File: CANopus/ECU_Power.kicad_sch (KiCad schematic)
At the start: 1 part

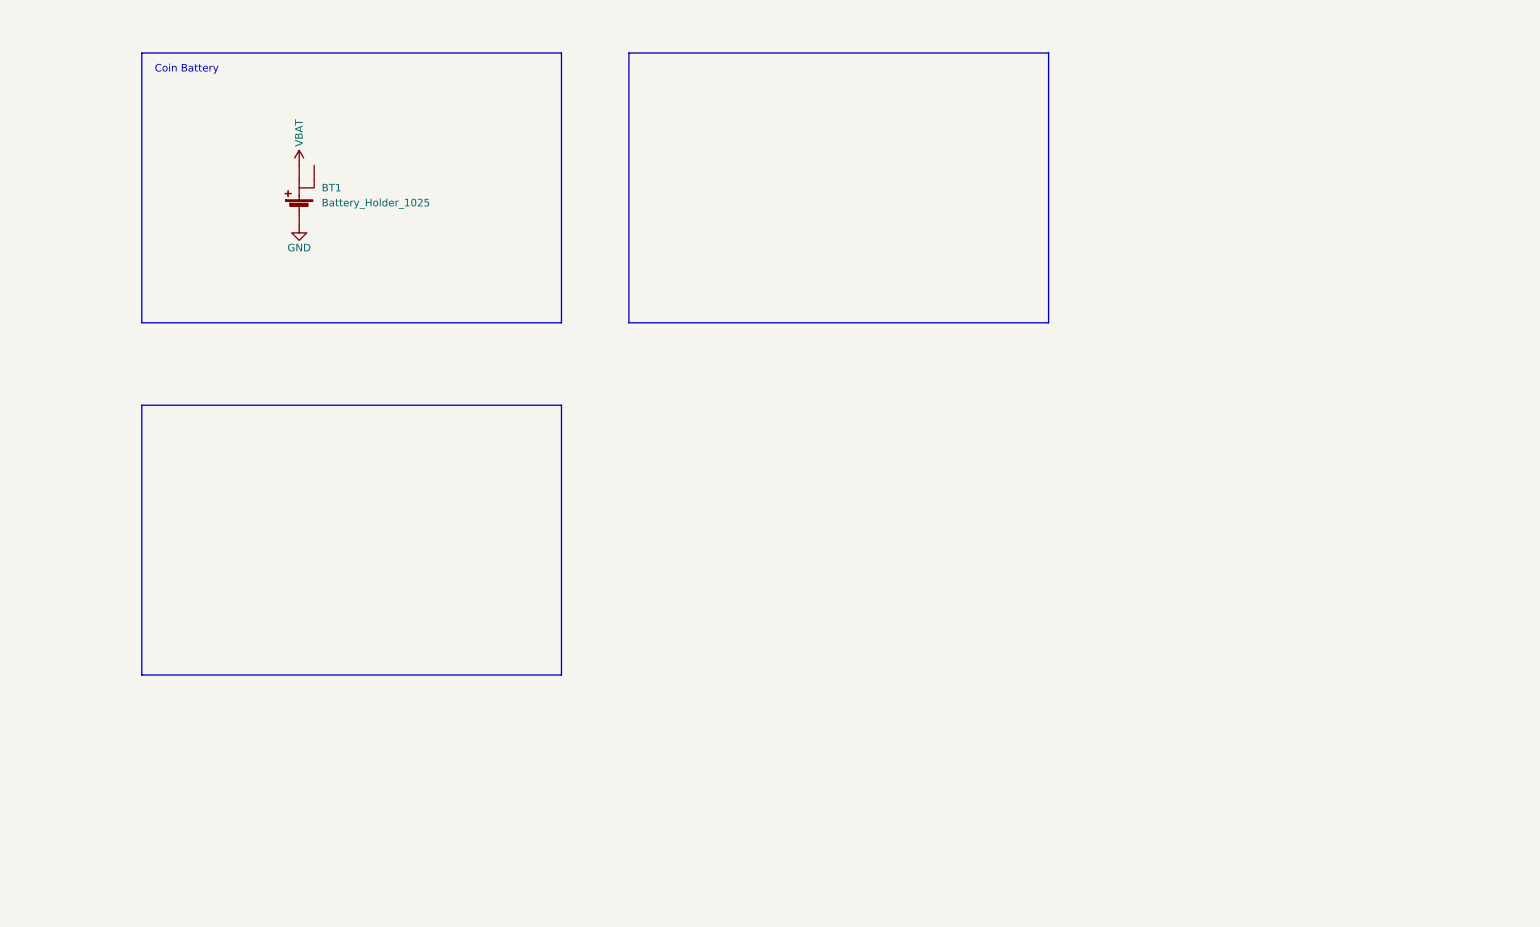
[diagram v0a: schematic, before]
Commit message: Alim
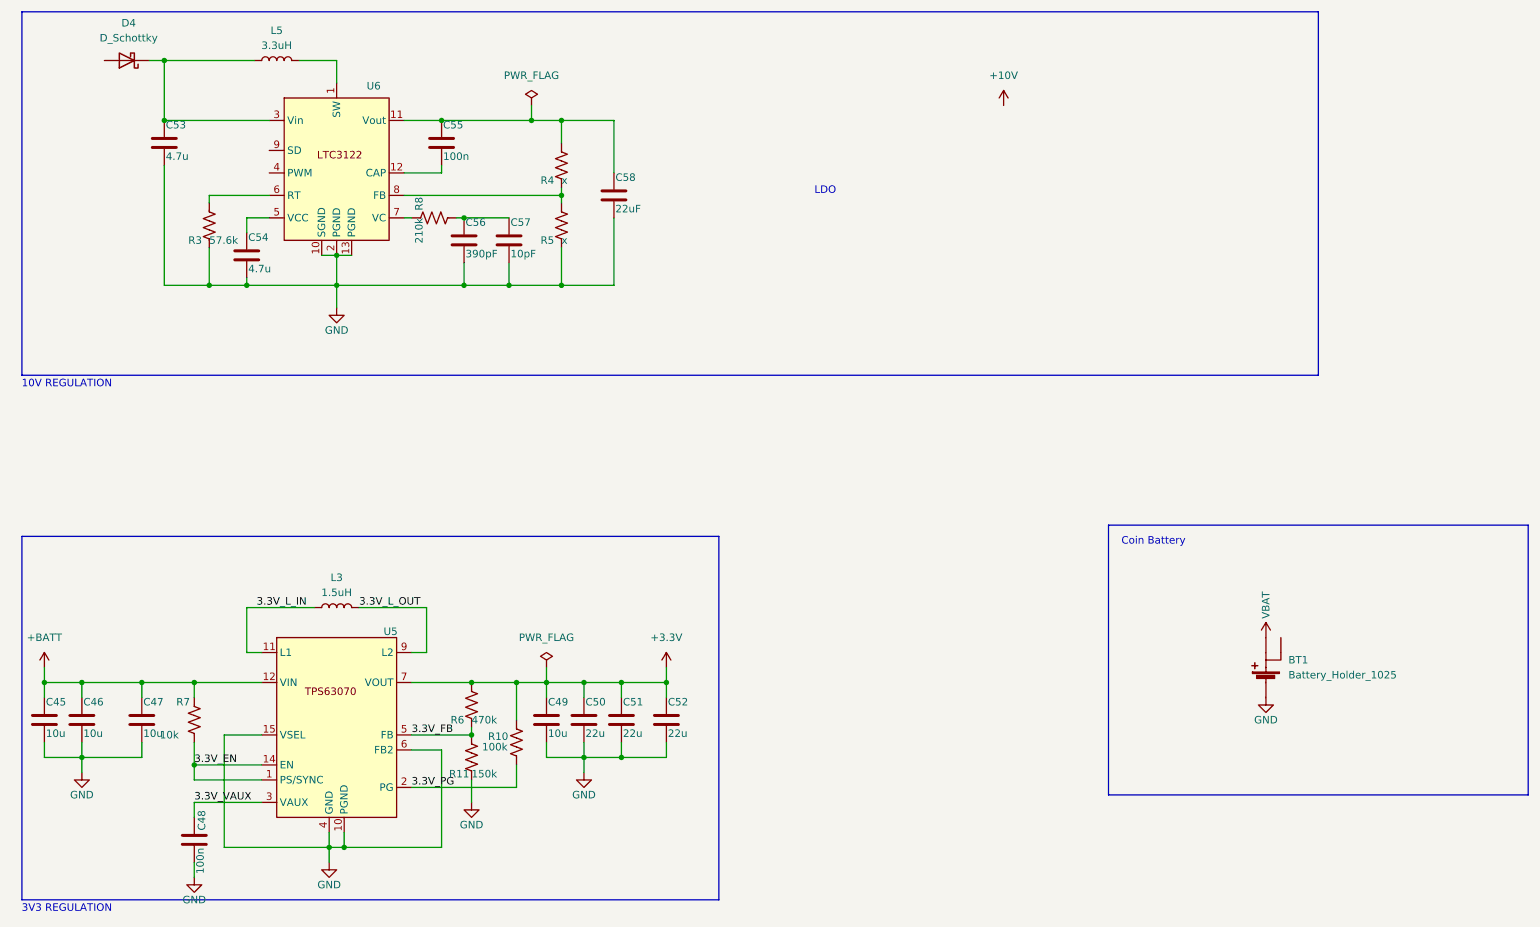
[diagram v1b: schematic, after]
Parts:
- added C45, C46: 10u, 0CSL_D1_V1:C0805_MAN, symbol Device:C
- added C47, C49: 10u, 0CSL_D1_V1:C0603_MAN, symbol Device:C
- added C48, C55: 100n, 0CSL_D1_V1:C0603_MAN, symbol Device:C
- added C50, C51, C52: 22u, 0CSL_D1_V1:C0805_MAN, symbol Device:C
- added C53, C54: 4.7u, 0CSL_D1_V1:C0805_MAN, symbol Device:C
- added C56: 390pF, 0CSL_D1_V1:C0805_MAN, symbol Device:C
- added C57: 10pF, 0CSL_D1_V1:C0805_MAN, symbol Device:C
- added C58: 22uF, 0CSL_D1_V1:C0805_MAN, symbol Device:C
- added D4: D_Schottky, symbol Device:D_Schottky
- added L3: 1.5uH, 0CSL_D1_V1:CUSTOM_BMRA000606301R5MA1, symbol Device:L
- added L5: 3.3uH, 0CSL_D1_V1:CUSTOM_BMRA000606301R5MA1, symbol Device:L
- added R10: 100k, 0CSL_D1_V1:R0603_MAN, symbol Device:R_US
- added R11: 150k, 0CSL_D1_V1:R0603_MAN, symbol Device:R_US
- added R3: 57.6k, 0CSL_D1_V1:R0603_MAN, symbol Device:R_US
- added R4, R5: x, 0CSL_D1_V1:R0603_MAN, symbol Device:R_US
- added R6: 470k, 0CSL_D1_V1:R0603_MAN, symbol Device:R_US
- added R7: 10k, 0CSL_D1_V1:R0603_MAN, symbol Device:R_US
- added R8: 210k, 0CSL_D1_V1:R0603_MAN, symbol Device:R_US
- added U5: ~, 0CSL_D1_V1:CUSTOM_VREG_TPS63070RNMR, symbol 0CSL_D1_V1:Custom_TPS63070
- added U6: ~, Footprint:MSOP-12_MSE, symbol 0CSL_D1_V1:LTC3122
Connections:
- net GND: now also C45.2, C46.2, C47.2, C48.1, C49.2, C50.2, C51.2, C52.2, C53.2, C54.2, C56.2, C57.2, C58.2, R11.2, R3.2, R5.2, U5.10 (PGND), U5.15 (VSEL), U5.4 (GND), U5.6 (FB2), U6.10 (SGND), U6.13 (PGND), U6.2 (PGND)
- new net: C54.1, U6.5 (VCC)
- new net: C56.1, C57.1, R8.1
- new net: C53.1, D4.1 (K), L5.1, U6.3 (Vin)
- new net: L5.2, U6.1 (SW)
- new net: C55.1, C58.1, R4.1, U6.11 (Vout)
- new net: C55.2, U6.12 (CAP)
- new net: R3.1, U6.6 (RT)
- new net: R8.2, U6.7 (VC)
- new net: R4.2, R5.1, U6.8 (FB)
- new net +3.3V: C49.1, C50.1, C51.1, C52.1, R10.1, R6.1, U5.7 (VOUT), U5.8 (VOUT)
- new net +BATT: C45.1, C46.1, C47.1, R7.1, U5.12 (VIN), U5.13 (VIN)
- new net 3.3V_EN: R7.2, U5.1 (PS/SYNC), U5.14 (EN)
- new net 3.3V_FB: R11.1, R6.2, U5.5 (FB)
- new net 3.3V_L_IN: L3.1, U5.11 (L1)
- new net 3.3V_L_OUT: L3.2, U5.9 (L2)
- new net 3.3V_PG: R10.2, U5.2 (PG)
- new net 3.3V_VAUX: C48.2, U5.3 (VAUX)
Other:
- note added: "10V REGULATION"
- note added: "3V3 REGULATION"
- note added: "LDO"
- moved on the sheet: BT1
